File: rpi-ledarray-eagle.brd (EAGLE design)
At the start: 33.5 x 19.2 mm, 27 parts

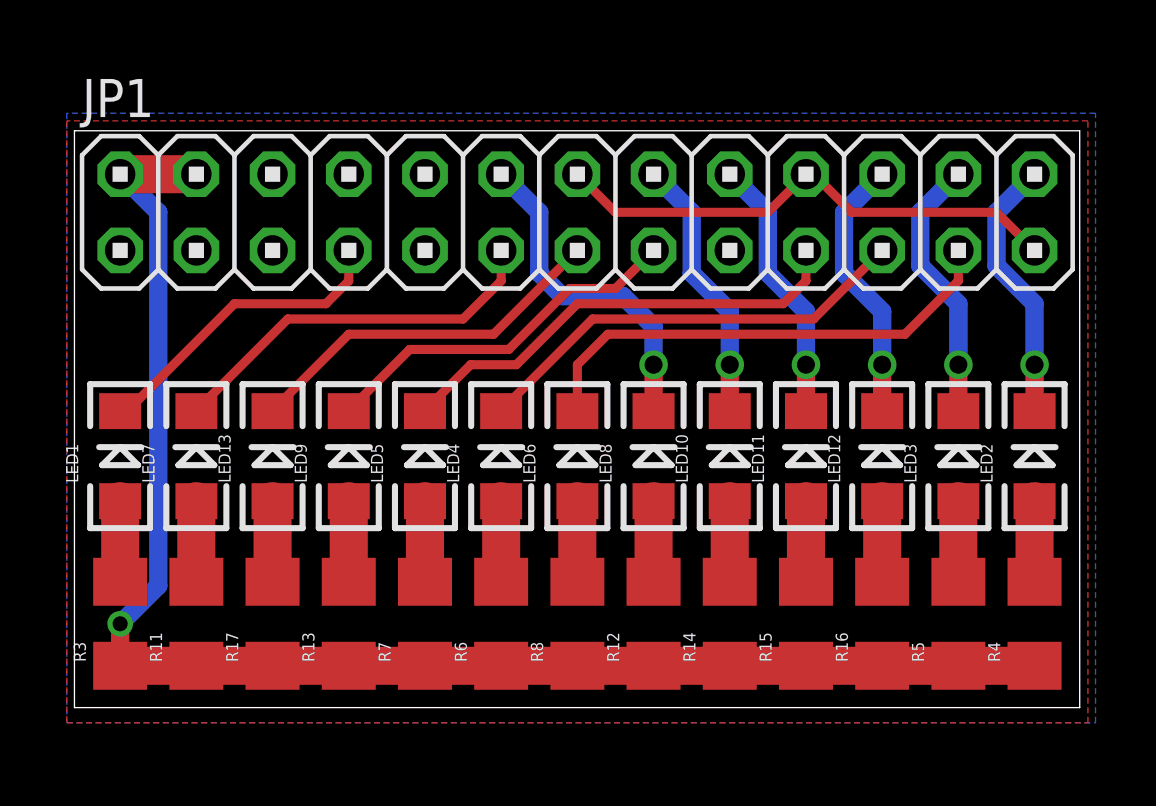
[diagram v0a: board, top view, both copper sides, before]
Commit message: First version finished
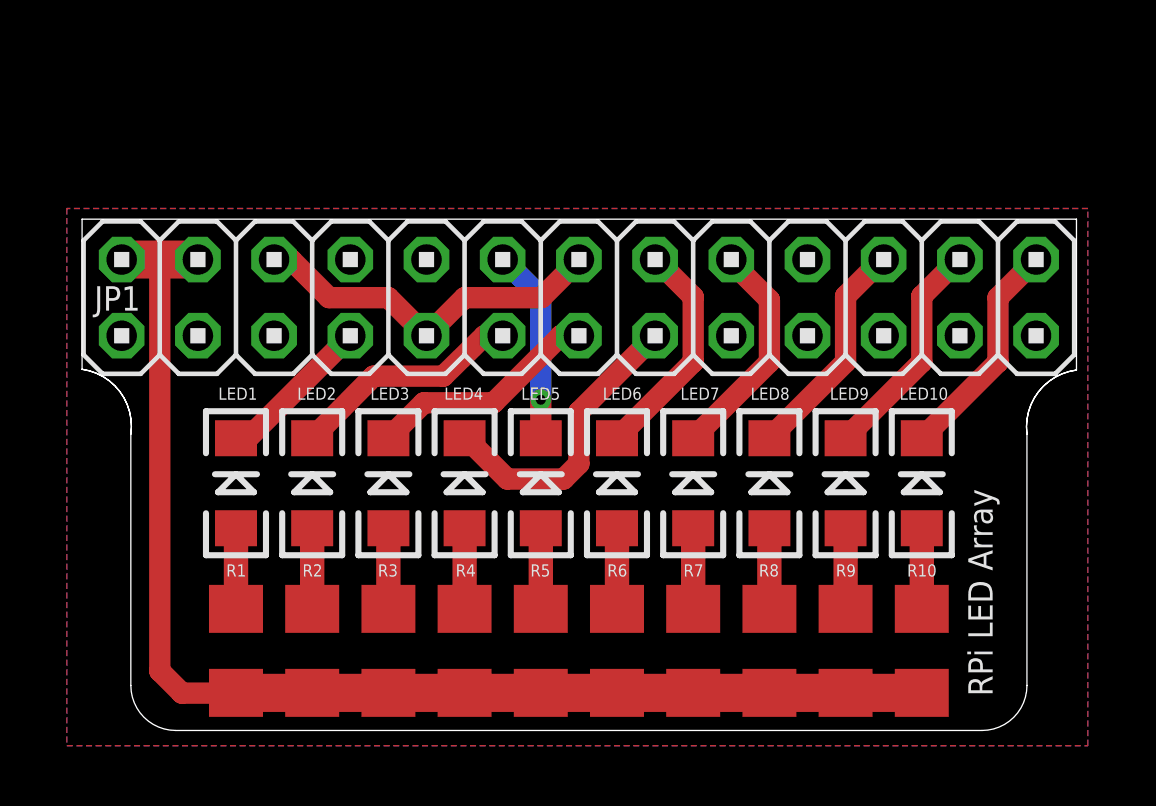
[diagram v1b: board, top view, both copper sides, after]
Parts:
- removed LED11, LED12, LED13: (no value), SparkFun:LED-1206
- removed R11, R12, R13, R14, R15, R16, R17: 270, SparkFun:1206
- added R1, R10, R2, R9: (no value), SparkFun:1206
- R3, R4, R5, R6, R7, R8: value 270 -> (none)
- moved LED2 24.1 mm to (7.67, 8.24)
- moved LED3 19.0 mm to (10.2, 8.24)
- moved R4 19.0 mm to (12.8, 2.65)
- moved LED7 16.6 mm to (20.4, 8.24)
- moved LED9 16.6 mm to (25.5, 8.24)
- moved R5 13.9 mm to (15.3, 2.65)
- moved R3 8.99 mm to (10.2, 2.65)
- moved R7 8.99 mm to (20.4, 2.65)
- moved LED10 6.46 mm to (28.0, 8.24)
- moved R8 6.46 mm to (22.9, 2.65)
- moved LED5 3.96 mm to (15.3, 8.24)
- moved LED1 3.96 mm to (5.13, 8.24)
- moved R6 3.96 mm to (17.8, 2.65)
- moved LED8 3.96 mm to (22.9, 8.24)
- moved JP1 2.85 mm to (16.6, 14.4)
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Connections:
- removed net N$16: LED12.A, R16.2
- removed net N$17: LED13.A, R17.2
- removed net N$7: LED5.A, R7.2
- removed net N$8: LED6.A, R8.2
- new net 3V3_1: JP1.1
- new net 3V3_2: JP1.17
- new net N$10: LED10.A, R10.2
- net 5V: now also R1.1, R10.1, R2.1, R9.1; no longer R11.1, R12.1, R13.1, R14.1, R15.1, R16.1, R17.1
- net GPIO10_MOSI: no longer LED5.C
- net GPIO11_SCLK: no longer LED6.C
- net GPIO17: now also LED2.C; no longer LED7.C
- net GPIO18: now also LED5.C; no longer LED8.C
- net GPIO22: now also LED4.C; no longer LED9.C
- net GPIO23: now also LED6.C; no longer LED10.C
- net GPIO24: now also LED7.C; no longer LED11.C
- net GPIO25: now also LED8.C; no longer LED12.C
- net GPIO27: now also LED3.C; no longer LED13.C
- net GPIO7: now also LED10.C; no longer LED2.C
- net GPIO8: now also LED9.C; no longer LED3.C
- net GPIO9_MISO: no longer LED4.C
- net N$11: now also LED9.A, R9.2; no longer LED7.A, R11.2
- net N$12: now also R8.2; no longer R12.2
- net N$13: now also LED7.A, R7.2; no longer LED9.A, R13.2
- net N$14: now also LED6.A, R6.2; no longer LED10.A, R14.2
- net N$15: now also LED5.A, R5.2; no longer LED11.A, R15.2
- net N$3: now also R1.2; no longer R3.2
- net N$4: now also R3.2; no longer R5.2
- net N$5: now also R2.2; no longer R4.2
- net N$6: now also R4.2; no longer R6.2
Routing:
- net GPIO11_SCLK: track 16.4 -> 0.00 mm
- net GPIO10_MOSI: track 15.5 -> 0.00 mm
- net GPIO9_MISO: track 14.9 -> 0.00 mm
- net 5V: track 50.5 -> 42.0 mm, vias 1 -> 0
- net GPIO17: track 13.0 -> 7.77 mm
- net GPIO4: track 10.4 -> 5.22 mm
- net GND: track 17.3 -> 12.3 mm
- net GPIO18: track 11.2 -> 6.50 mm
- net GPIO27: track 12.4 -> 7.76 mm
- net N$8: track 2.69 -> 0.00 mm
- net N$7: track 2.69 -> 0.00 mm
- net N$17: track 2.69 -> 0.00 mm
- net N$16: track 2.69 -> 0.00 mm
- net N$10: track 0.00 -> 2.69 mm
- net GPIO22: track 12.4 -> 9.90 mm
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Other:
- board size 33.5 x 19.2 mm -> 33.1 x 17 mm
- board text added: "R. Nugent prizepony.us"
- board text added: "RPi LED Array"
